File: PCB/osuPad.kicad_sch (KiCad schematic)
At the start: 8 parts, among them J1 OLED_128x32, U1 MCU_Seeed_XIAO_RP2040

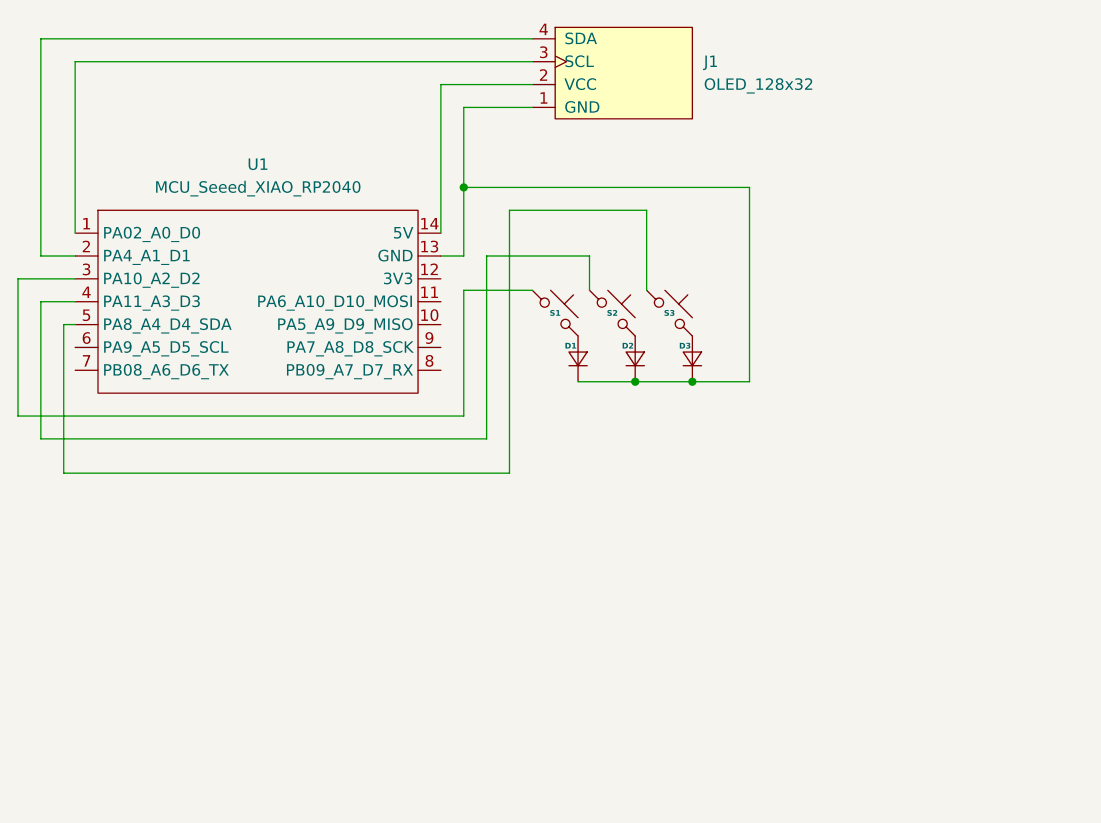
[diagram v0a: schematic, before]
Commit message: update pcb, case, and readme
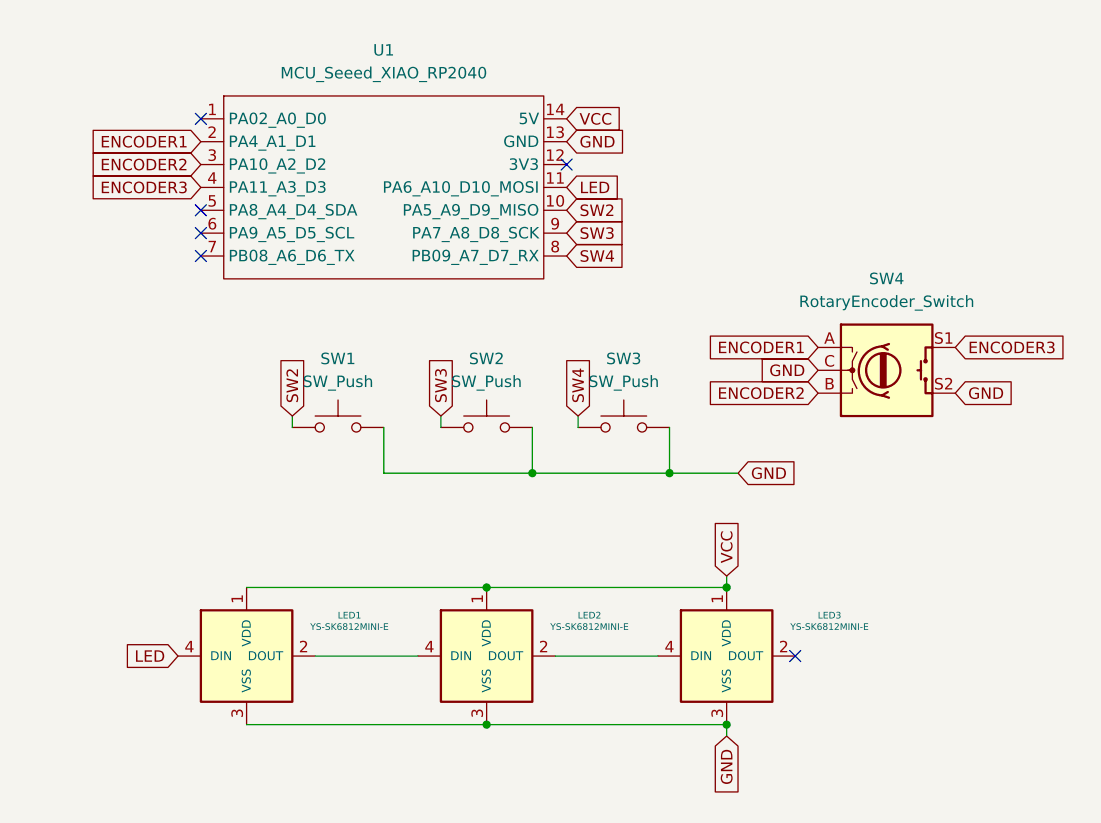
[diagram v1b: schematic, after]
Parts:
- removed D1, D2, D3: ~, ScottoKeebs_Components:Diode_DO-35, symbol ScottoKeebs:Placeholder_Diode
- removed J1: OLED_128x32, ScottoKeebs_Components:OLED_128x32, symbol ScottoKeebs:OLED_128x32
- removed S1, S2, S3: ~, ScottoKeebs_MX:MX_PCB_1.00u, symbol ScottoKeebs:Placeholder_Keyswitch
- added LED1, LED2, LED3: YS-SK6812MINI-E, kbd:YS-SK6812MINI-E, symbol kbd:YS-SK6812MINI-E
- added SW1, SW2, SW3: SW_Push, ScottoKeebs_Hotswap:Hotswap_MX_1.00u, symbol Switch:SW_Push
- added SW4: RotaryEncoder_Switch, Rotary_Encoder:RotaryEncoder_Alps_EC11E-Switch_Vertical_H20mm, symbol Device:RotaryEncoder_Switch
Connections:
- net SW2: now reaches U1.10 (PA5_A9_D9_MISO)
- net SW2: now also SW1.1
- net LED: now reaches U1.11 (PA6_A10_D10_MOSI)
- net LED: now also LED1.4 (DIN)
- net GND: now reaches U1.13 (GND)
- net GND: now also LED1.3 (VSS), LED2.3 (VSS), LED3.3 (VSS), SW1.2, SW2.2, SW3.2, SW4.C, SW4.S2
- net VCC: now reaches U1.14 (5V)
- net VCC: now also LED1.1 (VDD), LED2.1 (VDD), LED3.1 (VDD)
- net ENCODER1: now reaches U1.2 (PA4_A1_D1)
- net ENCODER1: now also SW4.A
- net ENCODER2: now reaches U1.3 (PA10_A2_D2)
- net ENCODER2: now also SW4.B
- net ENCODER3: now reaches U1.4 (PA11_A3_D3)
- net ENCODER3: now also SW4.S1
- net SW4: now reaches U1.8 (PB09_A7_D7_RX)
- net SW4: now also SW3.1
- net SW3: now reaches U1.9 (PA7_A8_D8_SCK)
- net SW3: now also SW2.1
- new net: LED2.2 (DOUT), LED3.4 (DIN)
- new net: LED1.2 (DOUT), LED2.4 (DIN)
- no-connect marks 0 -> 6
